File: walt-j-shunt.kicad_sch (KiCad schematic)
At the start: 39 parts, among them Q1 NMOS, Q2 PNP, Q3 PNP, U1 ${SIM.PARAMS}

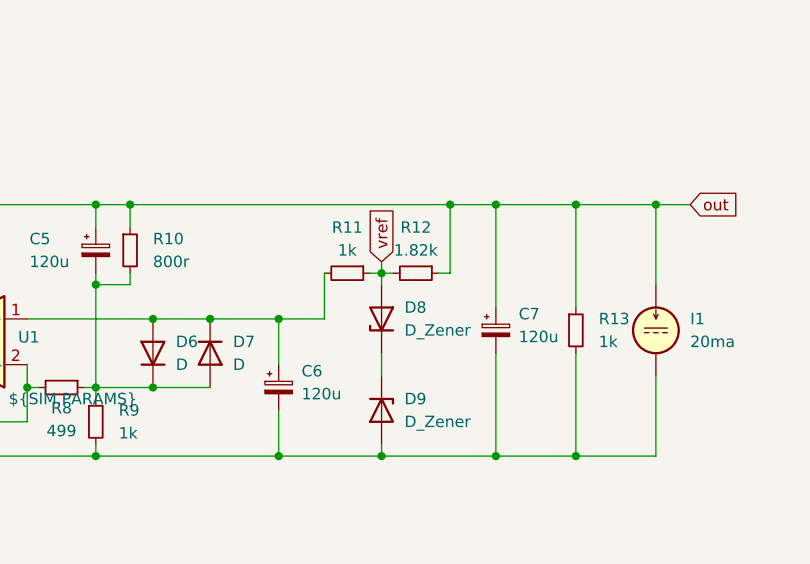
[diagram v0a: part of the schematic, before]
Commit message: footprint placeholders
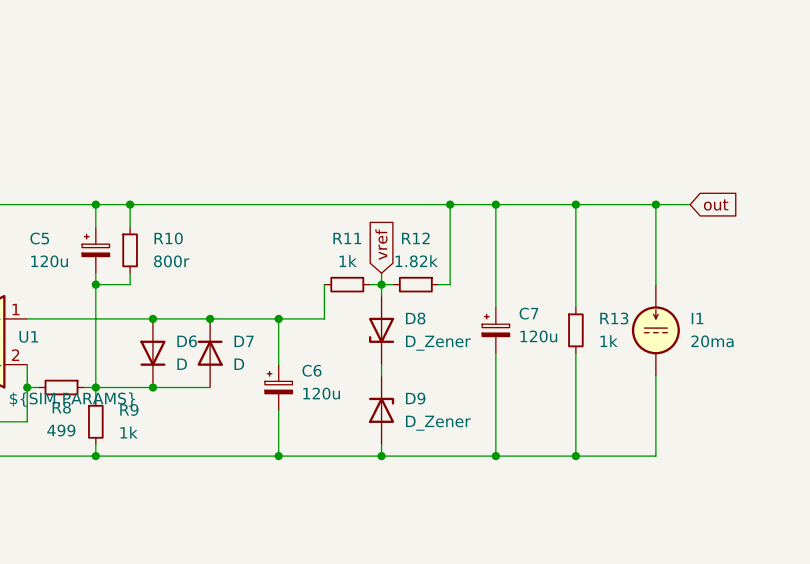
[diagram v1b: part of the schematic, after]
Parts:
- C4: footprint (none) -> Capacitor_THT:CP_Radial_D5.0mm_P2.00mm
- D5: footprint (none) -> Diode_SMD:D_0805_2012Metric
- D6, D7: footprint (none) -> Diode_SMD:D_SMC
- D8, D9: footprint (none) -> Package_TO_SOT_SMD:SOT-23-3
- Q1: footprint (none) -> Package_TO_SOT_THT:TO-3P-3_Horizontal_TabDown
- U1: footprint (none) -> Package_SO:SOIC-8-1EP_3.9x4.9mm_P1.27mm_EP2.41x3.3mm
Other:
- moved on the sheet: D8, R11, R12
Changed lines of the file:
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@@
 	)
 	(junction
-		(at 213.36 93.98)
+		(at 226.06 86.36)
 		(diameter 0)
 		(color 0 0 0 0)
 	)
 	(junction
-		(at 226.06 86.36)
+		(at 127 86.36)
 		(diameter 0)
 		(color 0 0 0 0)
 	)
 	(junction
-		(at 127 86.36)
+		(at 213.36 95.25)
 		(diameter 0)
 		(color 0 0 0 0)
@@
 	(wire
 		(pts
-			(xy 213.36 93.98) (xy 213.36 95.25)
-		)
-		(stroke
-			(width 0)
-			(type default)
-		)
-	)
-	(wire
-		(pts
-			(xy 219.71 93.98) (xy 220.98 93.98)
+			(xy 219.71 95.25) (xy 220.98 95.25)
 		)
 		(stroke
@@
 	(wire
 		(pts
-			(xy 220.98 93.98) (xy 220.98 86.36)
+			(xy 220.98 95.25) (xy 220.98 86.36)
 		)
 		(stroke
@@
 	(wire
 		(pts
-			(xy 213.36 92.71) (xy 213.36 93.98)
-		)
-		(stroke
-			(width 0)
-			(type default)
-		)
-	)
-	(wire
-		(pts
 			(xy 180.34 106.68) (xy 181.61 106.68)
 		)
@@
 	(wire
 		(pts
-			(xy 207.01 93.98) (xy 207.01 99.06)
+			(xy 207.01 95.25) (xy 207.01 99.06)
 		)
 		(stroke
@@
 	(wire
 		(pts
-			(xy 213.36 93.98) (xy 214.63 93.98)
+			(xy 213.36 95.25) (xy 214.63 95.25)
 		)
 		(stroke
@@
 	(wire
 		(pts
-			(xy 213.36 102.87) (xy 213.36 105.41)
+			(xy 213.36 95.25) (xy 213.36 93.98)
+		)
+		(stroke
+			(width 0)
+			(type default)
+		)
+	)
+	(wire
+		(pts
+			(xy 213.36 104.14) (xy 213.36 105.41)
 		)
 		(stroke
@@
 	(wire
 		(pts
+			(xy 213.36 95.25) (xy 213.36 96.52)
+		)
+		(stroke
+			(width 0)
+			(type default)
+		)
+	)
+	(wire
+		(pts
 			(xy 83.82 86.36) (xy 88.9 86.36)
 		)
@@
 	(wire
 		(pts
-			(xy 212.09 93.98) (xy 213.36 93.98)
+			(xy 212.09 95.25) (xy 213.36 95.25)
 		)
 		(stroke
@@
 	(global_label "vref"
 		(shape input)
-		(at 213.36 92.71 90)
+		(at 213.36 93.98 90)
 		(fields_autoplaced yes)
 		(effects
@@
 		)
 		(property "Intersheetrefs" "${INTERSHEET_REFS}"
-			(at 213.36 86.1567 90)
+			(at 213.36 87.4267 90)
 			(effects
 				(font
@@
 	(symbol
 		(lib_id "Device:R_Small")
-		(at 209.55 93.98 270)
+		(at 209.55 95.25 270)
 		(unit 1)
 		(exclude_from_sim no)
@@
 		(fields_autoplaced yes)
 		(property "Reference" "R11"
-			(at 209.55 88.9 90)
+			(at 209.55 90.17 90)
 			(effects
 				(font
@@
 		)
 		(property "Value" "1k"
-			(at 209.55 91.44 90)
+			(at 209.55 92.71 90)
 			(effects
 				(font
@@
 		)
 		(property "Footprint" "Resistor_SMD:R_1206_3216Metric"
-			(at 209.55 93.98 0)
+			(at 209.55 95.25 0)
 			(effects
 				(font
@@
 		)
 		(property "Datasheet" "~"
-			(at 209.55 93.98 0)
+			(at 209.55 95.25 0)
 			(effects
 				(font
@@
 		)
 		(property "Description" "Resistor, small symbol"
-			(at 209.55 93.98 0)
+			(at 209.55 95.25 0)
 			(effects
 				(font
@@
 			)
 		)
-		(property "Footprint" ""
+		(property "Footprint" "Diode_SMD:D_SMC"
 			(at 194.31 102.87 0)
 			(effects
@@
 			)
 		)
-		(property "Footprint" ""
+		(property "Footprint" "Diode_SMD:D_SMC"
 			(at 187.96 102.87 0)
 			(effects
@@
 			)
 		)
-		(property "Footprint" ""
+		(property "Footprint" "Diode_SMD:D_0805_2012Metric"
 			(at 153.67 101.6 0)
 			(effects
@@
 			)
 		)
-		(property "Footprint" ""
+		(property "Footprint" "Package_TO_SOT_THT:TO-3P-3_Horizontal_TabDown"
 			(at 111.76 83.82 0)
 			(effects
@@
 			)
 		)
-		(property "Footprint" ""
+		(property "Footprint" "Package_TO_SOT_SMD:SOT-23-3"
 			(at 213.36 109.22 0)
 			(effects
@@
 	(symbol
 		(lib_id "Device:D_Zener")
-		(at 213.36 99.06 90)
+		(at 213.36 100.33 90)
 		(unit 1)
 		(exclude_from_sim no)
@@
 		(fields_autoplaced yes)
 		(property "Reference" "D8"
-			(at 215.9 97.7899 90)
+			(at 215.9 99.0599 90)
 			(effects
 				(font
@@
 		)
 		(property "Value" "D_Zener"
-			(at 215.9 100.3299 90)
+			(at 215.9 101.5999 90)
 			(effects
 				(font
@@
 			)
 		)
-		(property "Footprint" ""
-			(at 213.36 99.06 0)
+		(property "Footprint" "Package_TO_SOT_SMD:SOT-23-3"
+			(at 213.36 100.33 0)
 			(effects
 				(font
@@
 		)
 		(property "Datasheet" "~"
-			(at 213.36 99.06 0)
+			(at 213.36 100.33 0)
 			(effects
 				(font
@@
 		)
 		(property "Description" "Zener diode"
-			(at 213.36 99.06 0)
+			(at 213.36 100.33 0)
 			(effects
 				(font
@@
 		)
 		(property "Sim.Library" "/Users/cibo/Documents/spice/d.lib"
-			(at 213.36 99.06 0)
+			(at 213.36 100.33 0)
 			(effects
 				(font
@@
 		)
 		(property "Sim.Name" "BZX84C6V2L"
-			(at 213.36 99.06 0)
+			(at 213.36 100.33 0)
 			(effects
 				(font
@@
 		)
 		(property "Sim.Device" "D"
-			(at 213.36 99.06 0)
+			(at 213.36 100.33 0)
 			(effects
 				(font
@@
 		)
 		(property "Sim.Pins" "1=K 2=A"
-			(at 213.36 99.06 0)
+			(at 213.36 100.33 0)
 			(effects
 				(font
@@
 			)
 		)
-		(property "Footprint" ""
+		(property "Footprint" "Capacitor_THT:CP_Radial_D5.0mm_P2.00mm"
 			(at 161.29 110.49 0)
 			(effects
@@
 	(symbol
 		(lib_id "Device:R_Small")
-		(at 217.17 93.98 270)
+		(at 217.17 95.25 270)
 		(unit 1)
 		(exclude_from_sim no)
@@
 		(fields_autoplaced yes)
 		(property "Reference" "R12"
-			(at 217.17 88.9 90)
+			(at 217.17 90.17 90)
 			(effects
 				(font
@@
 		)
 		(property "Value" "1.82k"
-			(at 217.17 91.44 90)
+			(at 217.17 92.71 90)
 			(effects
 				(font
@@
 		)
 		(property "Footprint" "Resistor_SMD:R_1206_3216Metric"
-			(at 217.17 93.98 0)
+			(at 217.17 95.25 0)
 			(effects
 				(font
@@
 		)
 		(property "Datasheet" "~"
-			(at 217.17 93.98 0)
+			(at 217.17 95.25 0)
 			(effects
 				(font
@@
 		)
 		(property "Description" "Resistor, small symbol"
-			(at 217.17 93.98 0)
+			(at 217.17 95.25 0)
 			(effects
 				(font
@@
 			)
 		)
-		(property "Footprint" ""
+		(property "Footprint" "Package_SO:SOIC-8-1EP_3.9x4.9mm_P1.27mm_EP2.41x3.3mm"
 			(at 166.37 101.6 0)
 			(effects
